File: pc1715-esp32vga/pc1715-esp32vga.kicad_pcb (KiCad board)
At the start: 2 copper layers, 112 x 38 mm, 31 parts, among them J1001 IDC10_VIDEO_IN, J1002 VGAOUT, J1003 USB_B, J1004 KEYPAD, J1005 IDC16_VGAOUT, SW1001 RST, U1001 ESP32-S3-WROOM-1, U1002 LM1117MP-3.3

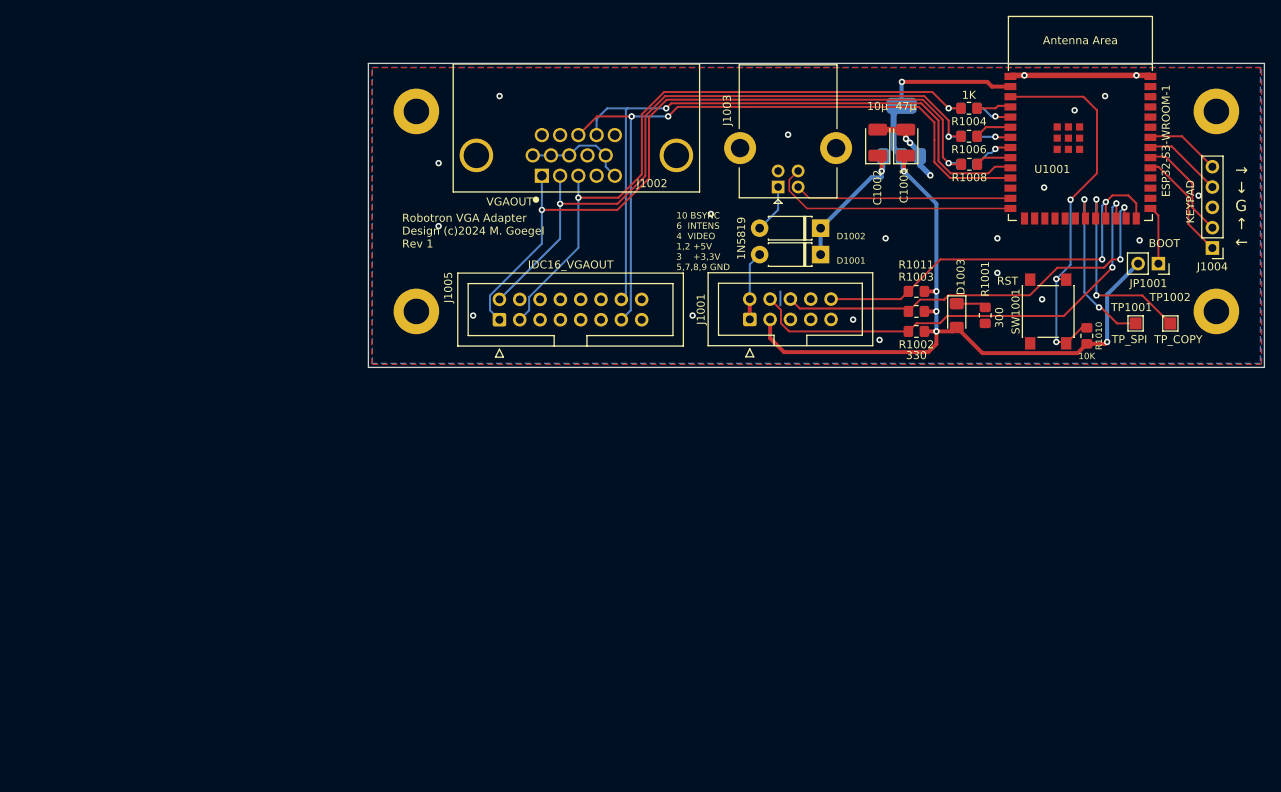
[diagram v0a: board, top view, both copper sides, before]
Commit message: Revision 2
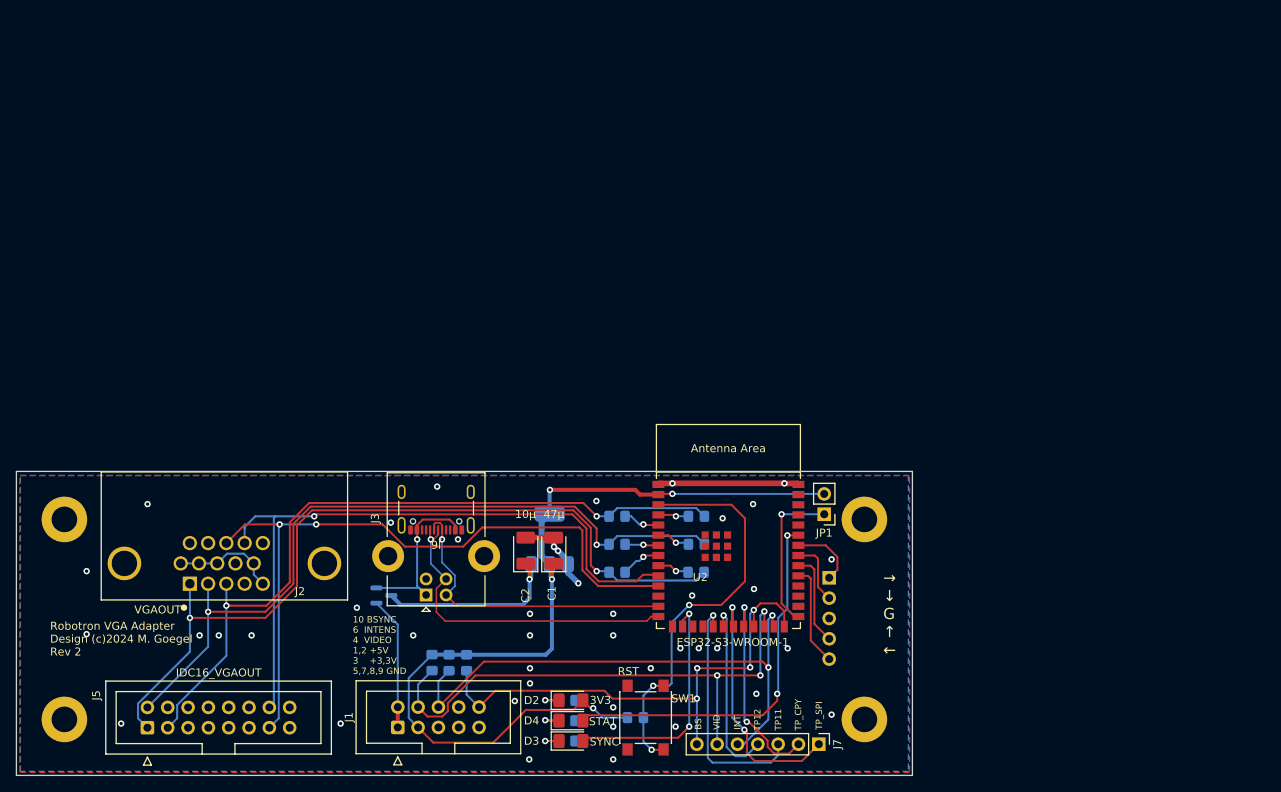
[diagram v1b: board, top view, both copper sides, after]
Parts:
- removed D1001, D1002: 1N5819, Diode_THT:D_DO-41_SOD81_P7.62mm_Horizontal
- removed D1003: LED, LED_SMD:LED_1206_3216Metric_Pad1.42x1.75mm_HandSolder
- removed R1001: 300, Resistor_SMD:R_0805_2012Metric_Pad1.20x1.40mm_HandSolder
- removed R1002, R1003, R1011: 330, Resistor_SMD:R_0805_2012Metric_Pad1.20x1.40mm_HandSolder
- removed TP1001: TP_SPI, TestPoint:TestPoint_Pad_1.5x1.5mm
- removed TP1002: TP_COPY, TestPoint:TestPoint_Pad_1.5x1.5mm
- added D1: BAT54C Uf 0,24V, Package_TO_SOT_SMD:SOT-23, B.Cu at (105.9, 115.5)
- added D2: 3V3, LED_SMD:LED_1206_3216Metric_Pad1.42x1.75mm_HandSolder, F.Cu at (129.3, 128.6)
- added D3: SYNC, LED_SMD:LED_1206_3216Metric_Pad1.42x1.75mm_HandSolder, F.Cu at (129.3, 133.7)
- added D4: STAT, LED_SMD:LED_1206_3216Metric_Pad1.42x1.75mm_HandSolder, F.Cu at (129.3, 131.2)
- added J6: USB_C_Receptacle_USB2.0_16P, Connector_USB:USB_C_Receptacle_GCT_USB4105-xx-A_16P_TopMnt_Horizontal, F.Cu at (112.5, 103.6)
- added J7: DBG, Connector_PinHeader_2.54mm:PinHeader_1x07_P2.54mm_Vertical, F.Cu at (160.3, 134.1)
- added R11: 330, Resistor_SMD:R_0805_2012Metric_Pad1.20x1.40mm_HandSolder, B.Cu at (112.0, 123.9)
- added R12: 330, Resistor_SMD:R_0805_2012Metric_Pad1.20x1.40mm_HandSolder, B.Cu at (114.1, 123.9)
- added R13: 330, Resistor_SMD:R_0805_2012Metric_Pad1.20x1.40mm_HandSolder, B.Cu at (116.3, 123.9)
- added R2: 330, Resistor_SMD:R_0805_2012Metric_Pad1.20x1.40mm_HandSolder, B.Cu at (128.8, 128.6)
- added R3: 330, Resistor_SMD:R_0805_2012Metric_Pad1.20x1.40mm_HandSolder, B.Cu at (128.8, 133.7)
- added R4: 330, Resistor_SMD:R_0805_2012Metric_Pad1.20x1.40mm_HandSolder, B.Cu at (128.8, 131.2)
- J4: renamed from J1004; footprint Connector_PinHeader_2.54mm:PinHeader_1x05_P2.54mm_Vertical -> Connector_PinSocket_2.54mm:PinSocket_1x05_P2.54mm_Horizontal; moved to B.Cu
- JP1: renamed from JP1001; footprint Connector_PinSocket_2.54mm:PinSocket_1x02_P2.54mm_Vertical -> Connector_PinHeader_2.54mm:PinHeader_1x02_P2.54mm_Vertical
- R1: renamed from R1010; moved to B.Cu
- R5: renamed from R1004; moved to B.Cu
- R7: renamed from R1006; moved to B.Cu
- R9: renamed from R1008; moved to B.Cu
- moved R1 73.9 mm to (137.4, 130.8), turned to 180 degrees
- moved SW1 71.5 mm to (138.7, 130.8)
- moved C1 67.4 mm to (127.2, 109.9)
- moved C2 67.4 mm to (123.7, 109.9)
- moved H1001 67.4 mm to (66.0, 106.0)
- moved H1002 67.4 mm to (66.0, 131.0)
- moved H1003 67.4 mm to (166.0, 106.0)
- moved H1004 67.4 mm to (166.0, 131.0)
- moved J1 67.4 mm to (107.7, 132.0)
- moved J2 67.4 mm to (86.0, 111.5)
- moved J3 67.4 mm to (111.2, 115.4)
- moved R10 67.4 mm to (135.1, 112.6)
- moved R6 67.4 mm to (135.1, 105.6)
- moved R8 67.4 mm to (135.1, 109.1)
- moved U1 67.4 mm to (126.7, 108.4)
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- renumbered C1001 to C1, C1002 to C2, J1001 to J1, J1002 to J2, J1003 to J3, J1005 to J5, R1009 to R10, R1005 to R6, R1007 to R8, SW1001 to SW1, U1002 to U1, U1001 to U2
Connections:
- net Net-(D1001-A) renamed /5V_VID
- J3 pad 1: Net-(D1002-A) -> /VBUS
- J4 pad 1: /K_LEFT -> /K_RIGHT
- J4 pad 2: /K_UP -> /K_DOWN
- J4 pad 4: /K_DOWN -> /K_UP
- J4 pad 5: /K_RIGHT -> /K_LEFT
- U2 pad 16: unconnected-(U1001-GPIO46-Pad16) -> Net-(D3-A)
- U2 pad 19: unconnected-(U1001-GPIO11/TOUCH11/ADC2_CH0/FSPID/FSPIIO5/SUBSPID-Pad19) -> /TP_11
- U2 pad 20: unconnected-(U1001-GPIO12/TOUCH12/ADC2_CH1/FSPICLK/FSPIIO6/SUBSPICLK-Pad20) -> /TP_12
- U2 pad 21: Net-(U1001-GPIO13/TOUCH13/ADC2_CH2/FSPIQ/FSPIIO7/SUBSPIQ) -> /TP_SPI
- U2 pad 22: Net-(U1001-GPIO14/TOUCH14/ADC2_CH3/FSPIWP/FSPIDQS/SUBSPIWP) -> /TP_CPY
- U2 pad 35: unconnected-(U1001-MTMS/GPIO42-Pad35) -> Net-(D4-A)
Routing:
- net Net-(D4-A): track 0.00 -> 47.9 mm, vias 0 -> 2
- net /TP_SPI: track 0.00 -> 31.5 mm, vias 0 -> 2
- net /TP_11: track 0.00 -> 30.3 mm, vias 0 -> 1
- net Net-(D3-A): track 0.00 -> 30.1 mm, vias 0 -> 2
- net /TP_CPY: track 0.00 -> 25.9 mm, vias 0 -> 2
- net Net-(U1001-GPIO14/TOUCH14/ADC2_CH3/FSPIWP/FSPIDQS/SUBSPIWP): track 25.0 -> 0.00 mm, vias 2 -> 0
- net /TP_12: track 0.00 -> 23.0 mm, vias 0 -> 1
- net Net-(U1001-GPIO13/TOUCH13/ADC2_CH2/FSPIQ/FSPIIO7/SUBSPIQ): track 22.0 -> 0.00 mm, vias 2 -> 0
- net /VBUS: track 0.00 -> 21.7 mm, vias 0 -> 1
- net /INTENS: track 52.6 -> 68.7 mm
- net /BSYNC: track 51.6 -> 65.5 mm, vias 2 -> 4
- net Net-(JP1-A): track 7.44 -> 19.3 mm, vias 0 -> 1
- net /USB_DN: track 27.2 -> 39.0 mm, vias 0 -> 1
- net /VIDEO: track 58.7 -> 69.8 mm, vias 2 -> 3
- net /GREEN: track 83.6 -> 94.6 mm
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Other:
- board text added: "BS"
- board text added: "INT"
- board text added: "J3"
- board text added: "Robotron VGA Adapter Design (c)2024 M. Goegel Rev 2"
- board text added: "TP11"
- board text added: "TP12"
- board text added: "TP_CPY"
- board text added: "TP_SPI"
- board text added: "VID"
- board text removed: "Robotron VGA Adapter Design (c)2024 M. Goegel Rev 1"
